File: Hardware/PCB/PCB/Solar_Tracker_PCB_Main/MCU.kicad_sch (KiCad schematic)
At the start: 22 parts, among them IC1 ESP32-S3-WROOM-1-N4R8, IC5 LM1117MPX-3.3_NOPB, J1 1729076, J2 USB4940-00-A, J3 1729076, J4 1977223-1, J5 1977223-1, J6 1729076

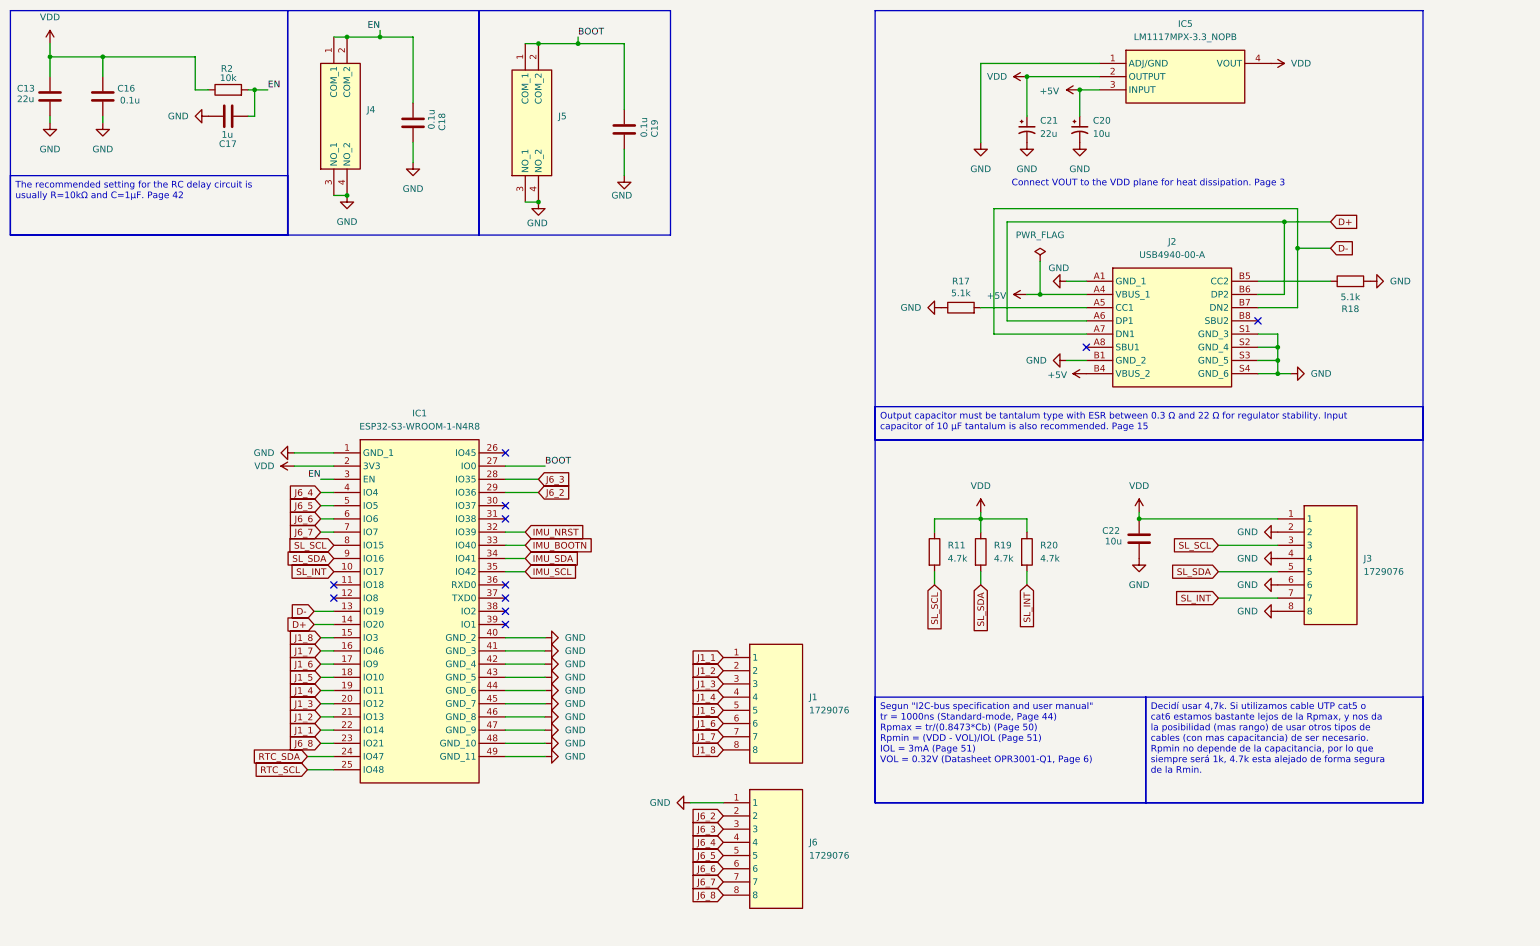
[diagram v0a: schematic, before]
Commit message: Agregue conectores JST
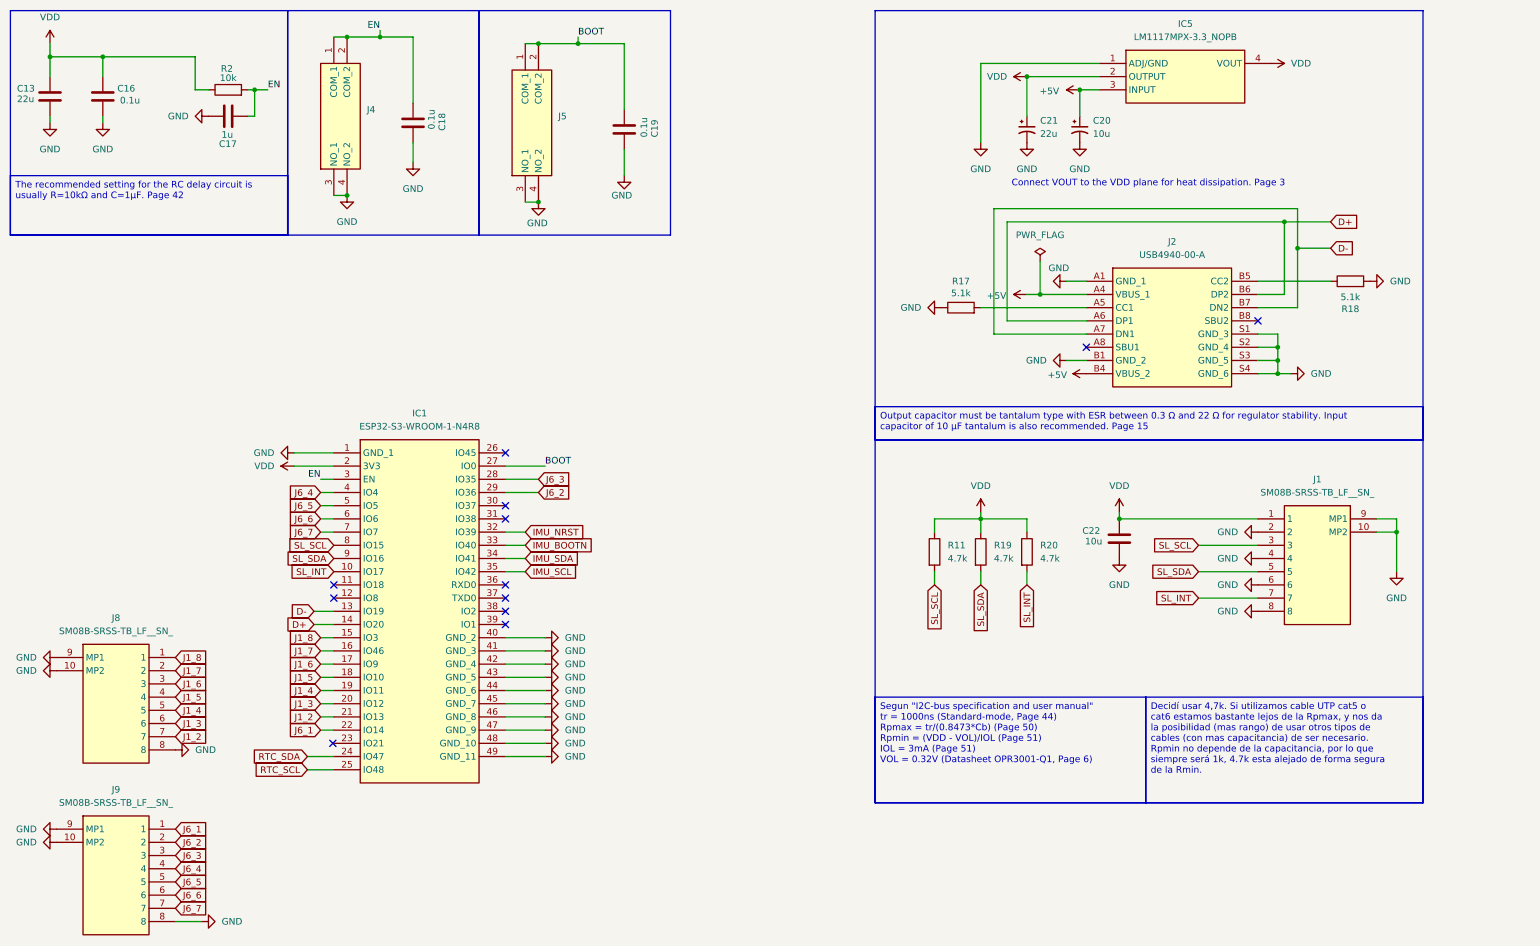
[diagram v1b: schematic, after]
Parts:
- removed J1, J3, J6: 1729076, 1729076:1729076, symbol 1729076:1729076
- added J1, J8, J9: SM08B-SRSS-TB_LF__SN_, SM08B:SM08BSRSSTBLFSN, symbol SM08B-SRSS-TB_LF__SN_:SM08B-SRSS-TB_LF__SN_
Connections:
- net GND: now also J1.10 (MP2), J1.2, J1.4, J1.6, J1.8, J1.9 (MP1), J8.10 (MP2), J8.8, J8.9 (MP1), J9.10 (MP2), J9.8, J9.9 (MP1)
- net J1_2: now also J8.7
- net J1_3: now also J8.6
- net J1_4: now also J8.5
- net J1_5: now also J8.4
- net J1_6: now also J8.3
- net J1_7: now also J8.2
- net J1_8: now also J8.1
- net J6_2: now also J9.2
- net J6_3: now also J9.3
- net J6_4: now also J9.4
- net J6_5: now also J9.5
- net J6_6: now also J9.6
- net J6_7: now also J9.7
- net SL_INT: now also J1.7
- net SL_SCL: now also J1.3
- net SL_SDA: now also J1.5
- net VDD: now also J1.1
- net J1_1 renamed J6_1
- net J6_1: now also J9.1
- net J6_8: no longer names the net of IC1.23 (IO21)
- no-connect marks 11 -> 12
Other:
- moved on the sheet: C22
